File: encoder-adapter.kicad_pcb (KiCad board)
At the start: 2 copper layers, 23 x 23 mm, 3 parts, among them J1 Conn_01x04, J2 Conn_01x03, J3 Conn_01x04

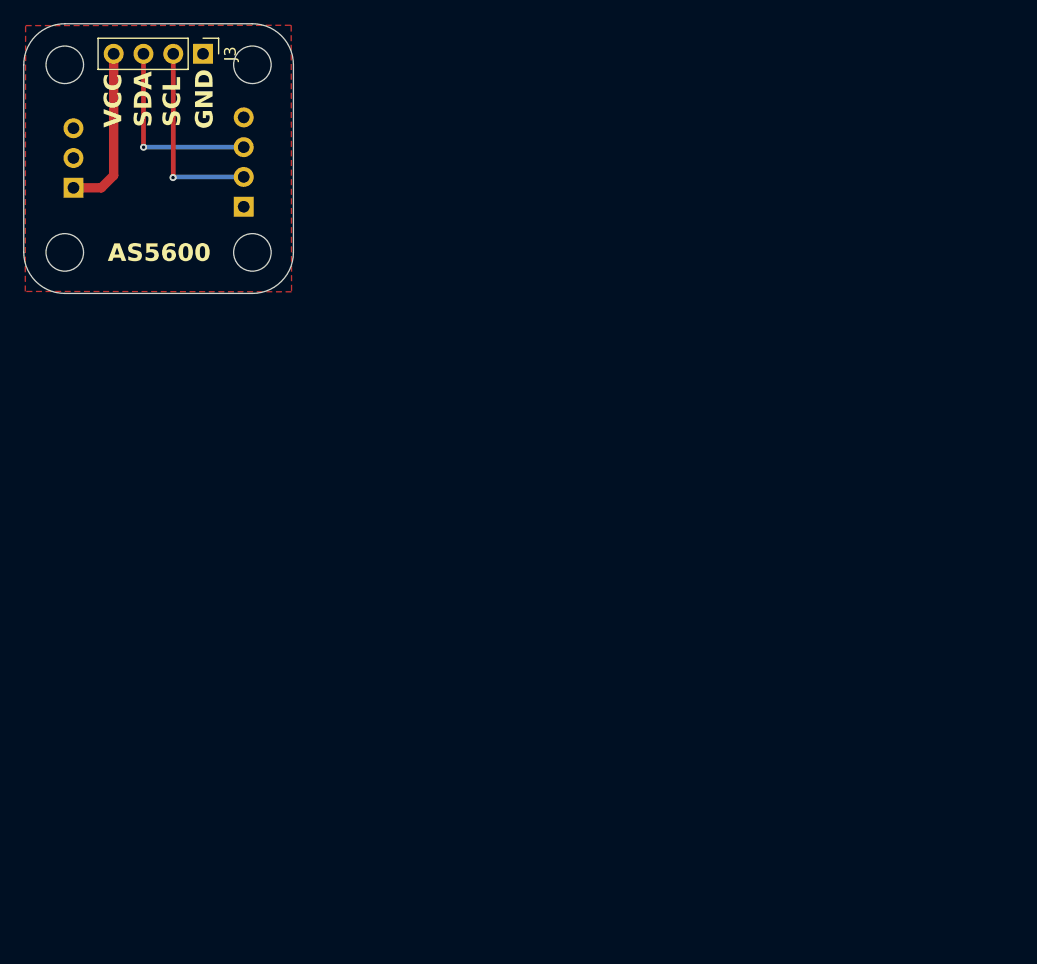
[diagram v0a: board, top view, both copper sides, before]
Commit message: add encoder photo
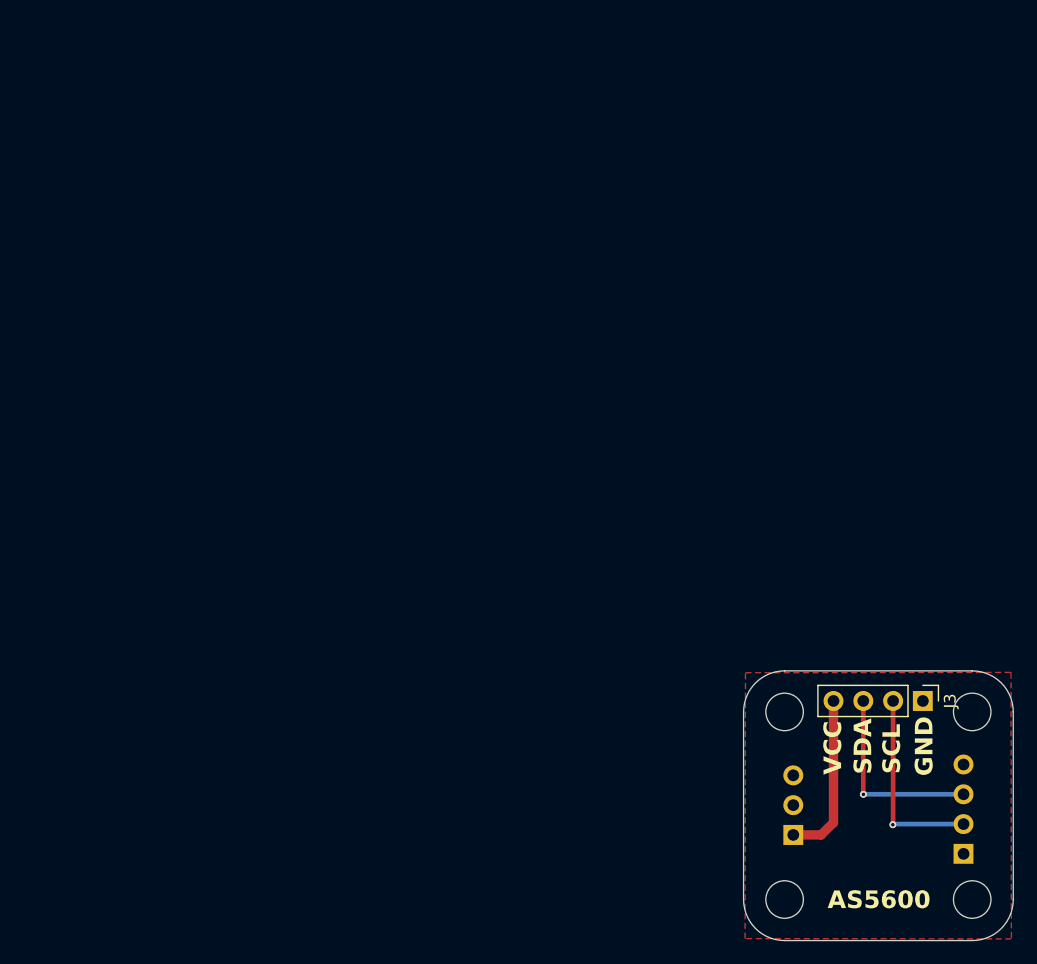
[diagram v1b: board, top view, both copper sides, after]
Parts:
- moved J1 82.6 mm to (76.7, 67.3)
- moved J2 82.6 mm to (62.1, 65.7)
- moved J3 82.6 mm to (73.2, 54.3)
